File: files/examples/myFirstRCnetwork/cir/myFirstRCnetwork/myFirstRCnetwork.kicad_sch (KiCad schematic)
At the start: 4 parts

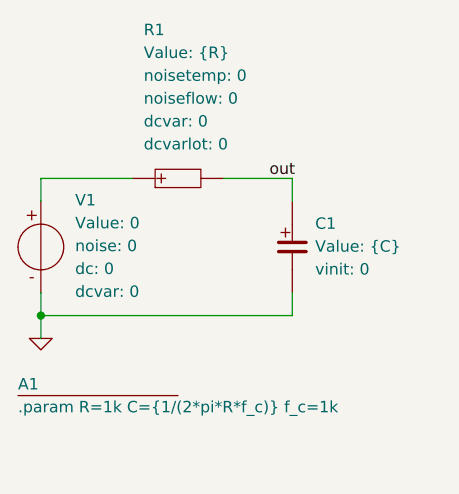
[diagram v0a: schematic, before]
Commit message: This is now SLiCAP Version 3
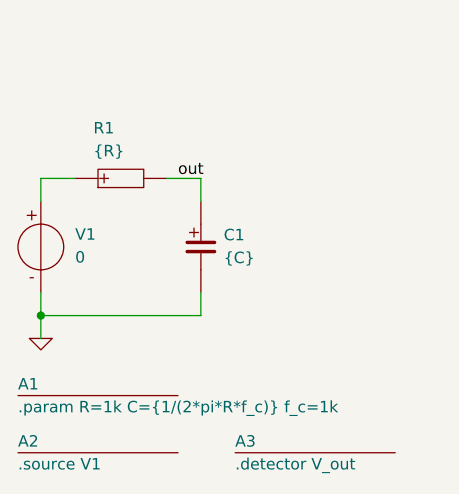
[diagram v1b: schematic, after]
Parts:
- added A2, A3: ~, symbol SLiCAP:Command
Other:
- moved on the sheet: C1, R1
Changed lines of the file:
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@@
-(kicad_sch (version 20230121) (generator eeschema)
-  (paper "A4")
-  (title_block
-    (title "myFirstRCnetwork")
-  )
+(kicad_sch
+	(version 20231120)
+	(generator "eeschema")
+	(generator_version "8.0")
+	(paper "A4")
+	(title_block
+		(title "myFirstRCnetwork")
+	)
